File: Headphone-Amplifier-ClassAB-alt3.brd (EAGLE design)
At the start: 40.6 x 17.8 mm, 17 parts, among them T1 2N3904, T2 2N3904, T3 2N3906

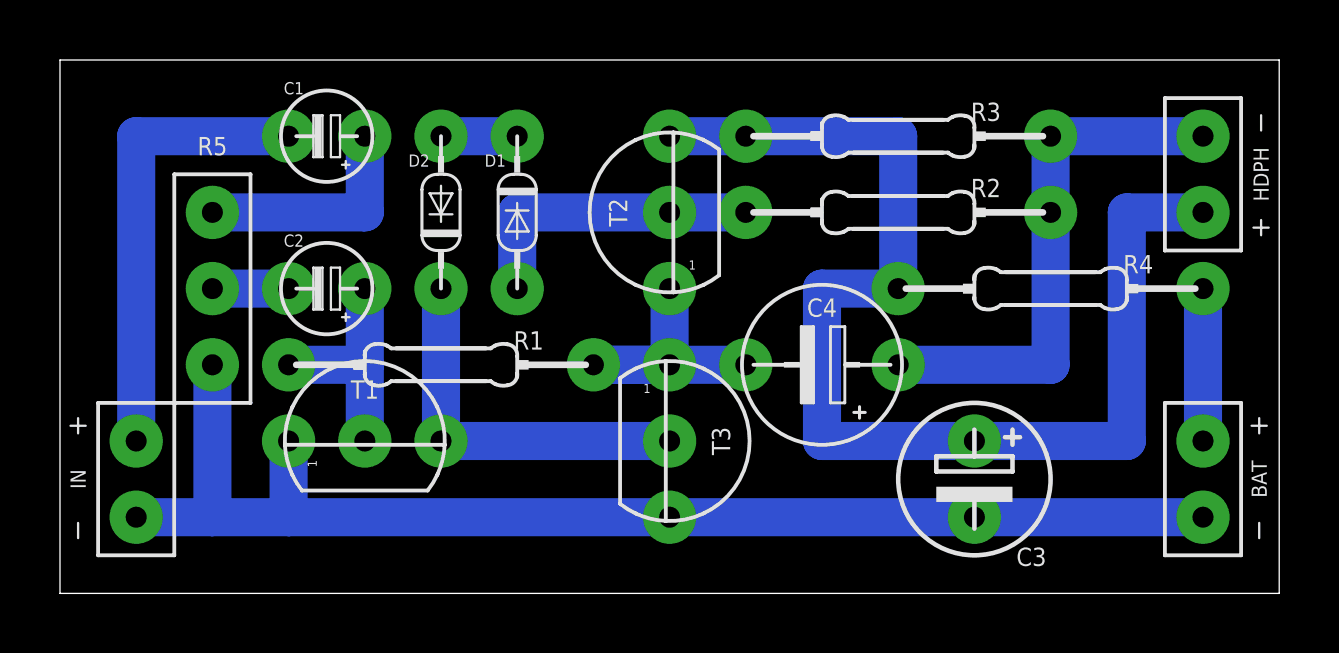
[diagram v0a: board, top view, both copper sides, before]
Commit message: ...
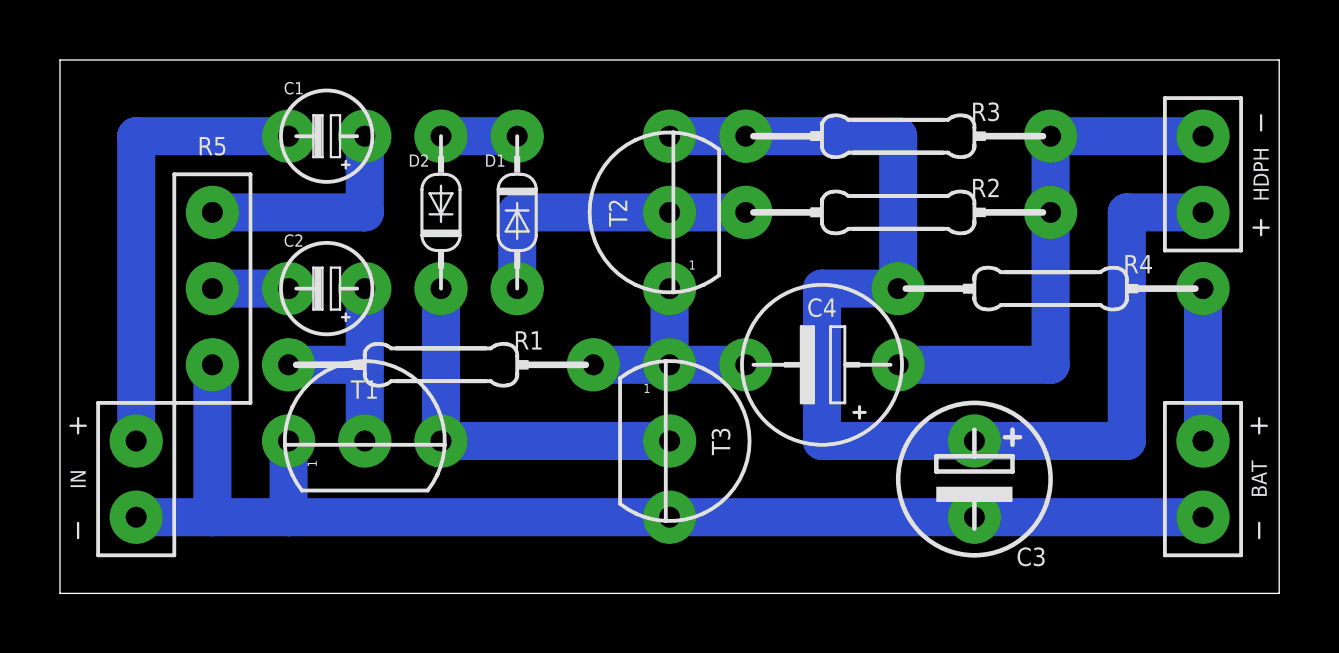
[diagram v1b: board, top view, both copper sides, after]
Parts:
- BAT: value SPAD+-+- -> (none)
- HDPH, IN: value SPAD+--+ -> (none)
- T2: value 2N3904 -> S8050
- T3: value 2N3906 -> (none)
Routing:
- net N$4: track 10.2 -> 7.62 mm
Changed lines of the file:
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@@
       <layer number="44" name="Drills" color="7" fill="1" visible="no" active="yes" />
       <layer number="45" name="Holes" color="7" fill="1" visible="yes" active="yes" />
-      <layer number="46" name="Milling" color="3" fill="1" visible="no" active="yes" />
-      <layer number="47" name="Measures" color="7" fill="1" visible="no" active="yes" />
-      <layer number="48" name="Document" color="7" fill="1" visible="no" active="yes" />
-      <layer number="49" name="Reference" color="7" fill="1" visible="no" active="yes" />
+      <layer number="46" name="Milling" color="3" fill="1" visible="yes" active="yes" />
+      <layer number="47" name="Measures" color="7" fill="1" visible="yes" active="yes" />
+      <layer number="48" name="Document" color="7" fill="1" visible="yes" active="yes" />
+      <layer number="49" name="Reference" color="7" fill="1" visible="yes" active="yes" />
       <layer number="51" name="tDocu" color="6" fill="1" visible="yes" active="yes" />
       <layer number="52" name="bDocu" color="7" fill="1" visible="no" active="yes" />
@@
       </autorouter>
       <elements>
-        <element name="BAT" library="pad" package="SPAD+-" value="SPAD+-+-" x="38.1" y="3.81" />
+        <element name="BAT" library="pad" package="SPAD+-" value="" x="38.1" y="3.81" />
         <element name="C1" library="c" package="E2,5-3" value="4.7uF" x="8.89" y="15.24" rot="R180" />
         <element name="C2" library="c" package="E2,5-3" value="4.7uF" x="8.89" y="10.16" rot="R180" />
@@
         <element name="D1" library="d" package="DO34-5-V" value="1N4148" x="15.24" y="12.7" />
         <element name="D2" library="d" package="DO34-5V" value="1N4148" x="12.7" y="12.7" />
-        <element name="HDPH" library="pad" package="SPAD-+" value="SPAD+--+" x="38.1" y="13.97" rot="R180" />
-        <element name="IN" library="pad" package="SPAD-+" value="SPAD+--+" x="2.54" y="3.81" />
+        <element name="HDPH" library="pad" package="SPAD-+" value="" x="38.1" y="13.97" rot="R180" />
+        <element name="IN" library="pad" package="SPAD-+" value="" x="2.54" y="3.81" />
         <element name="R1" library="r" package="0204/10" value="100k" x="12.7" y="7.62" />
         <element name="R2" library="r" package="0204/10" value="330" x="27.94" y="12.7" />
@@
         <element name="R5" library="r" package="CONN-3P" value="100k" x="5.08" y="10.16" />
         <element name="T1" library="t" package="TO92" value="2N3904" x="10.16" y="5.08" rot="R90" />
-        <element name="T2" library="t" package="TO92" value="2N3904" x="20.32" y="12.7" rot="R180" />
-        <element name="T3" library="t" package="TO92" value="2N3906" x="20.32" y="5.08" />
+        <element name="T2" library="t" package="TO92" value="S8050" x="20.32" y="12.7" rot="R180" />
+        <element name="T3" library="t" package="TO92" value="" x="20.32" y="5.08" />
       </elements>
       <signals>
@@
           <contactref element="D2" pad="C" />
           <contactref element="T1" pad="3" />
+          <wire x1="12.7" y1="10.16" x2="12.7" y2="5.08" width="1.27" layer="16" />
           <contactref element="T3" pad="2" />
-          <wire x1="12.7" y1="10.16" x2="12.7" y2="5.08" width="1.27" layer="16" />
           <wire x1="12.7" y1="5.08" x2="20.32" y2="5.08" width="1.27" layer="16" />
         </signal>
@@
           <contactref element="T2" pad="1" />
           <contactref element="T3" pad="1" />
-          <wire x1="22.86" y1="7.62" x2="17.78" y2="7.62" width="1.27" layer="16" />
-          <wire x1="17.78" y1="7.62" x2="20.32" y2="7.62" width="1.27" layer="16" />
+          <wire x1="20.32" y1="7.62" x2="17.78" y2="7.62" width="1.27" layer="16" />
           <wire x1="20.32" y1="7.62" x2="20.32" y2="10.16" width="1.27" layer="16" />
+          <wire x1="20.32" y1="7.62" x2="22.86" y2="7.62" width="1.27" layer="16" />
         </signal>
         <signal name="N$5">
@@
           <contactref element="R5" pad="1" />
           <contactref element="IN" pad="1" />
-          <contactref element="T3" pad="3" />
           <wire x1="2.54" y1="2.54" x2="5.08" y2="2.54" width="1.27" layer="16" />
           <wire x1="5.08" y1="7.62" x2="5.08" y2="2.54" width="1.27" layer="16" />
           <wire x1="5.08" y1="2.54" x2="7.62" y2="2.54" width="1.27" layer="16" />
           <wire x1="7.62" y1="5.08" x2="7.62" y2="2.54" width="1.27" layer="16" />
+          <wire x1="30.48" y1="2.54" x2="38.1" y2="2.54" width="1.27" layer="16" />
+          <contactref element="T3" pad="3" />
           <wire x1="7.62" y1="2.54" x2="20.32" y2="2.54" width="1.27" layer="16" />
-          <wire x1="30.48" y1="2.54" x2="20.32" y2="2.54" width="1.27" layer="16" />
-          <wire x1="30.48" y1="2.54" x2="38.1" y2="2.54" width="1.27" layer="16" />
+          <wire x1="20.32" y1="2.54" x2="30.48" y2="2.54" width="1.27" layer="16" />
         </signal>
         <signal name="N$9">
